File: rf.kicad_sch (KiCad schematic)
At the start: 10 parts, among them Q1 2N7002

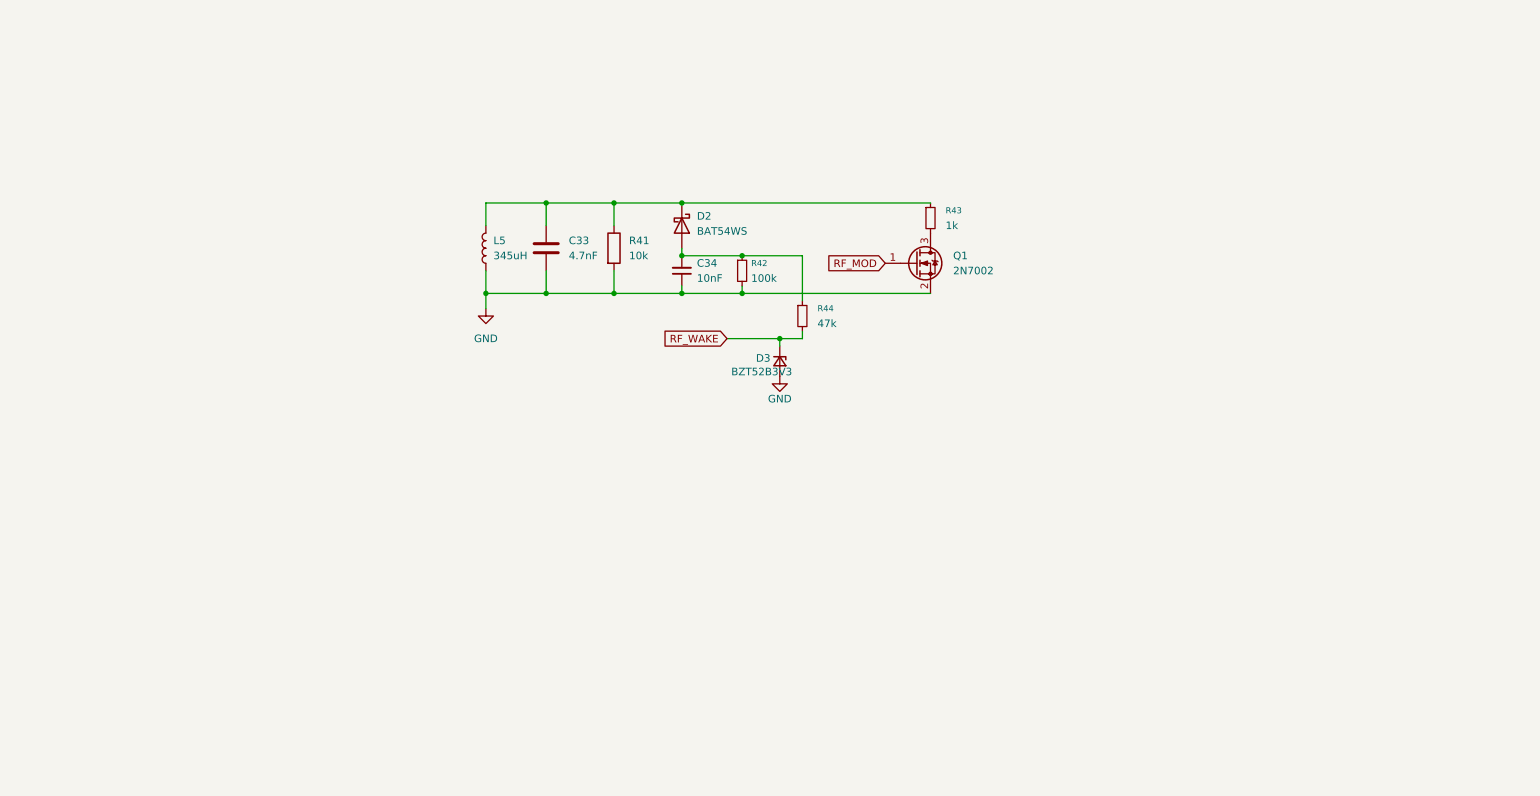
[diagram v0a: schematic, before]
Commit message: finish up everything but nfc
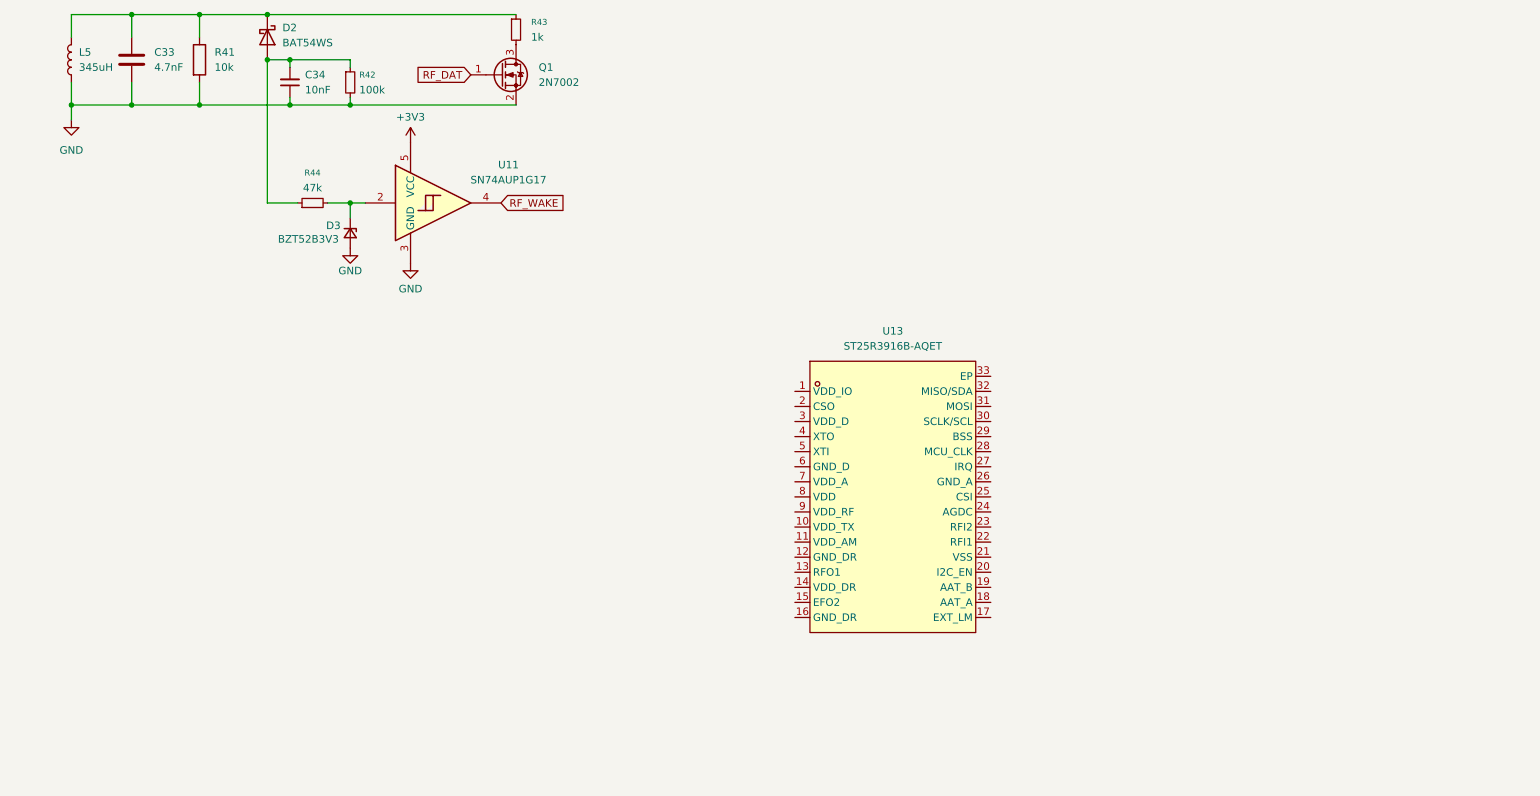
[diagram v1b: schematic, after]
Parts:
- added U11: SN74AUP1G17, Package_TO_SOT_SMD:Diodes_SOT-553, symbol 74xGxx:74LVC1G17
- added U13: ST25R3916B-AQET, ST25R3916B-AQET:QFN-32_L5.0-W5.0-P0.50-TL-EP3.5, symbol ST25R3916B-AQET:ST25R3916B-AQET
- C33: LCSC Part (none) -> C1538
- C34: footprint (none) -> Capacitor_SMD:C_0402_1005Metric; LCSC Part (none) -> C15195
- L5: footprint (none) -> custom_footprints:Generic_Solder_Pads_2P; now left out of the parts list
- Q1: LCSC Part (none) -> C8545
- R41: footprint (none) -> Resistor_SMD:R_0402_1005Metric; LCSC Part (none) -> C25744
- R42: footprint (none) -> Resistor_SMD:R_0402_1005Metric; LCSC Part (none) -> C25741
- R43: footprint (none) -> Resistor_SMD:R_0603_1608Metric; LCSC Part (none) -> C21190
- R44: footprint (none) -> Resistor_SMD:R_0402_1005Metric; LCSC Part (none) -> C25792
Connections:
- net GND: now also U11.3 (GND)
- net RF_WAKE: now also U11.4; no longer D3.1 (K), R44.2
- net RF_MOD renamed RF_DAT
- new net: D3.1 (K), R44.2, U11.2
- new net +3V3: U11.5 (VCC)
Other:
- moved on the sheet: C33, C34, D2, L5, Q1, R41, R42, R43, R44

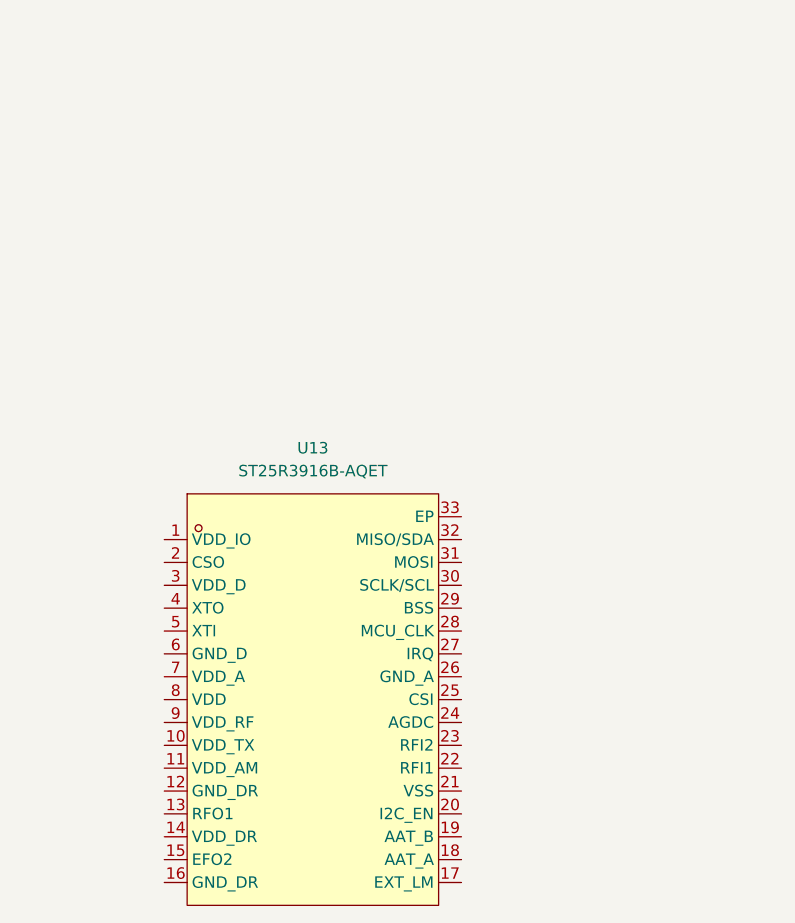
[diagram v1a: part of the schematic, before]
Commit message: progress
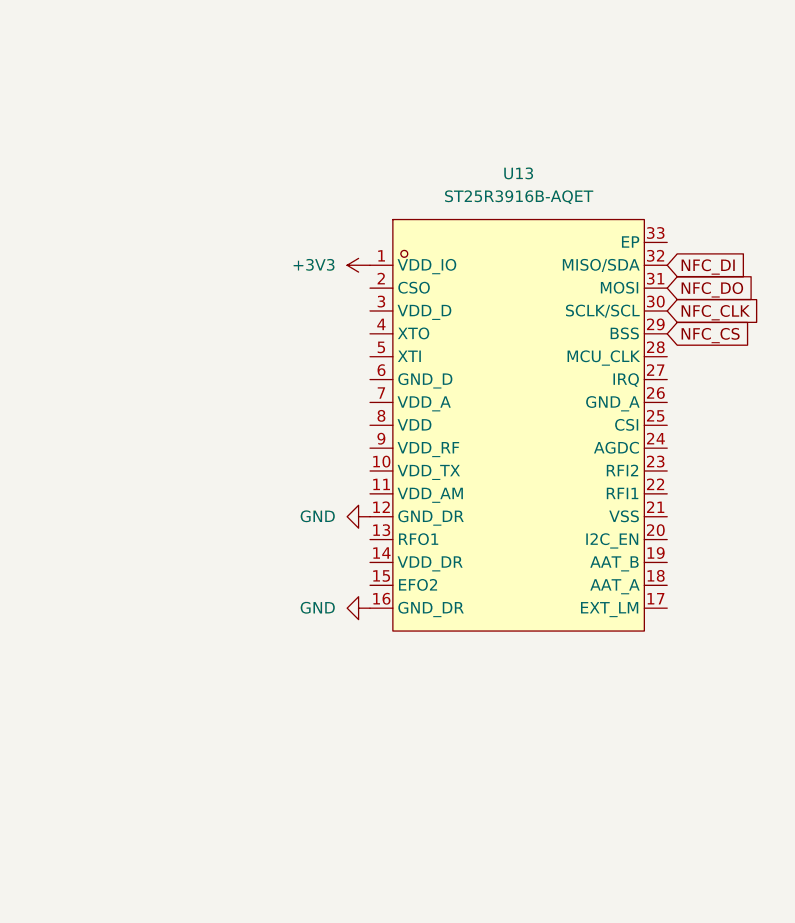
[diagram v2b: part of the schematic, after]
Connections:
- net +3V3: now also U13.1 (VDD_IO)
- net GND: now also U13.12 (GND_DR), U13.16 (GND_DR)
- net NFC_CS: now reaches U13.29 (BSS)
- net NFC_CLK: now reaches U13.30 (SCLK/SCL)
- net NFC_DO: now reaches U13.31 (MOSI)
- net NFC_DI: now reaches U13.32 (MISO/SDA)
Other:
- moved on the sheet: U13

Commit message: push changes before removing fuel gauge
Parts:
- L5: now in the parts list
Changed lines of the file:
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@@
 		(unit 1)
 		(exclude_from_sim no)
-		(in_bom no)
+		(in_bom yes)
 		(on_board yes)
 		(dnp no)

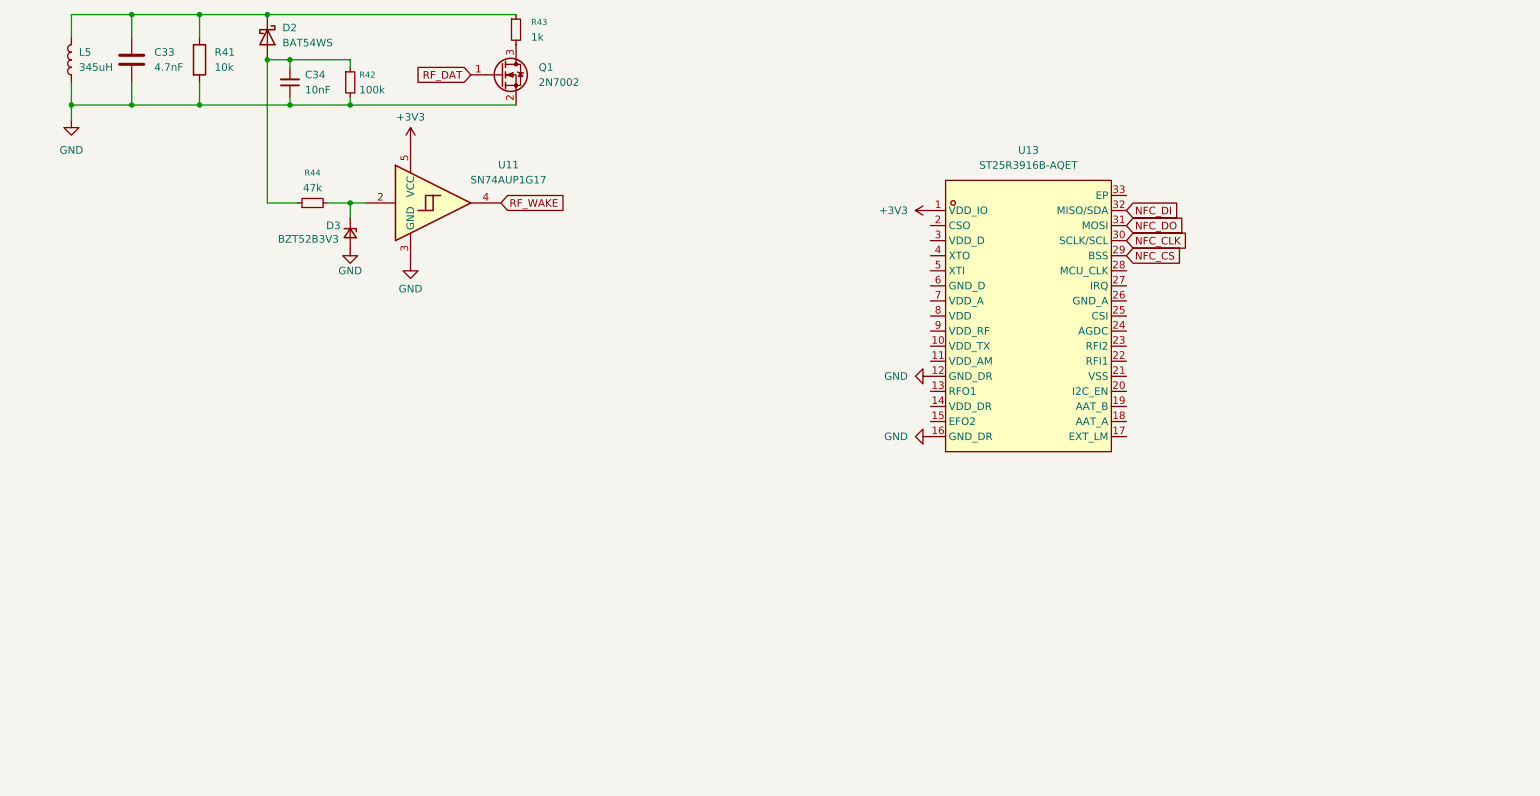
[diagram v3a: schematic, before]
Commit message: hopefully final schematic before splitting out
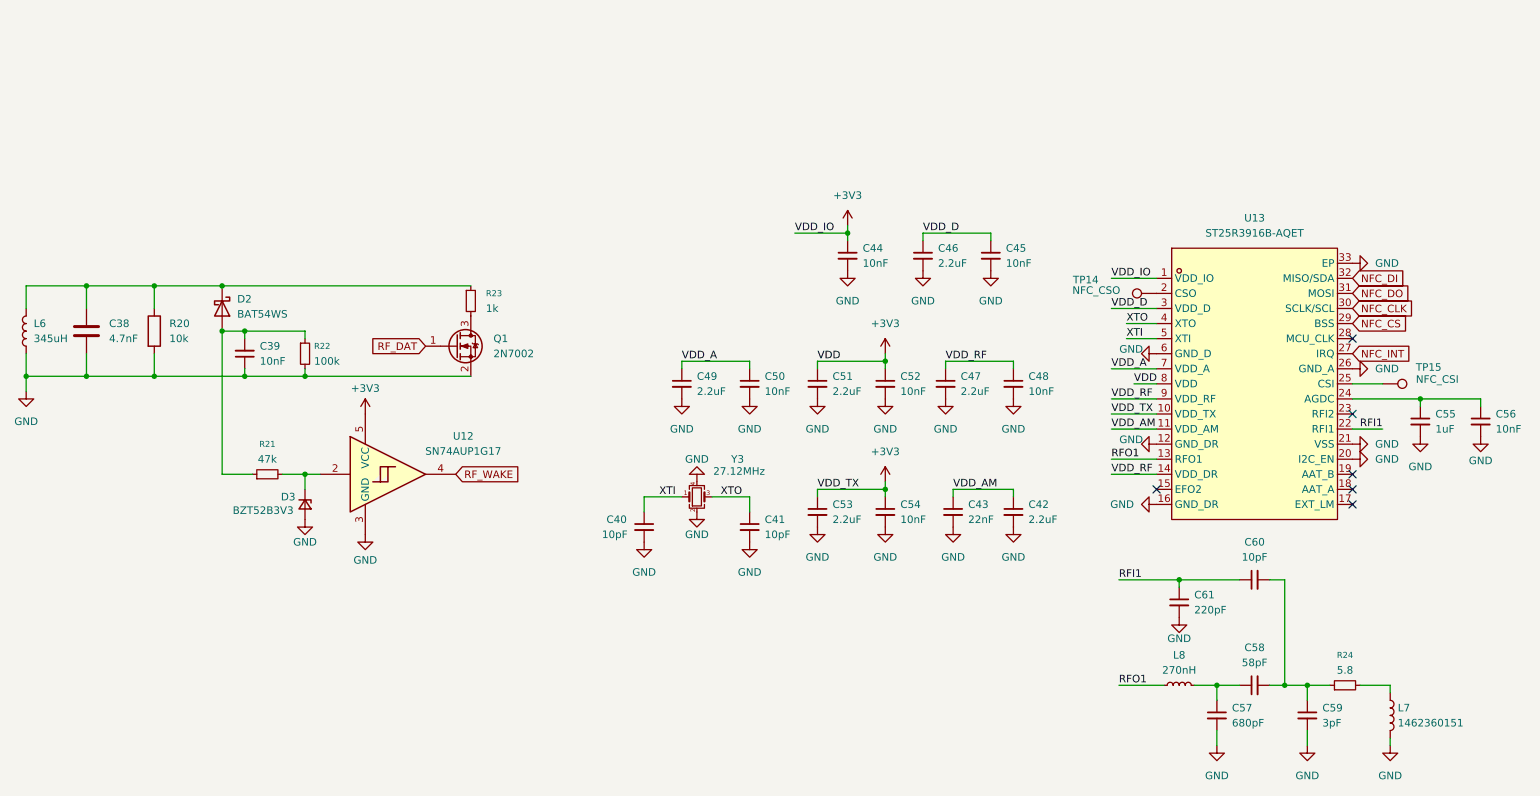
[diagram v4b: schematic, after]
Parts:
- added C40, C41, C60: 10pF, Capacitor_SMD:C_0402_1005Metric, symbol Device:C_Small
- added C42, C46, C47, C49, C51, C53: 2.2uF, Capacitor_SMD:C_0402_1005Metric, symbol Device:C_Small
- added C43: 22nF, Capacitor_SMD:C_0402_1005Metric, symbol Device:C_Small
- added C44, C45, C48, C50, C52, C54, C56: 10nF, Capacitor_SMD:C_0402_1005Metric, symbol Device:C_Small
- added C55: 1uF, Capacitor_SMD:C_0402_1005Metric, symbol Device:C_Small
- added C57: 680pF, Capacitor_SMD:C_0402_1005Metric, symbol Device:C_Small
- added C58: 58pF, Capacitor_SMD:C_0402_1005Metric, symbol Device:C_Small
- added C59: 3pF, Capacitor_SMD:C_0402_1005Metric, symbol Device:C_Small
- added C61: 220pF, Capacitor_SMD:C_0402_1005Metric, symbol Device:C_Small
- added L7: 1462360151, custom_footprints:Generic_Solder_Pads_2P, symbol Device:L
- added L8: 270nH, Inductor_SMD:L_0603_1608Metric, symbol Device:L_Small
- added R24: 5.8, Resistor_SMD:R_0402_1005Metric, symbol Device:R_Small
- added TP14: NFC_CSO, TestPoint:TestPoint_Pad_D1.0mm, symbol Connector:TestPoint
- added TP15: NFC_CSI, TestPoint:TestPoint_Pad_D1.0mm, symbol Connector:TestPoint
- added Y3: 27.12MHz, Crystal:Crystal_SMD_2016-4Pin_2.0x1.6mm, symbol Device:Crystal_GND24_Small
- L6: renamed from L5; now left out of the parts list
- renumbered C33 to C38, C34 to C39, R41 to R20, R44 to R21, R42 to R22, R43 to R23, U11 to U12
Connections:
- net +3V3: now also U13.10 (VDD_TX), U13.8 (VDD), C44.1, C51.1, C52.1, C53.1, C54.1
- net GND: now also U13.20 (I2C_EN), U13.21 (VSS), U13.26 (GND_A), U13.33 (EP), U13.6 (GND_D), C40.2, C41.2, C42.2, C43.2, C44.2, C45.2, C46.2, C47.2, C48.2, C49.2, C50.2, C51.2, C52.2, C53.2, C54.2, C55.2, C56.2, C57.2, C59.2, C61.2, L7.2, Y3.2, Y3.4
- net VDD_AM: now reaches U13.11 (VDD_AM)
- net VDD_AM: now also C42.1, C43.1
- net RFO1: now reaches U13.13 (RFO1)
- net RFO1: now also L8.1
- net VDD_RF: now reaches U13.14 (VDD_DR)
- net VDD_RF: now also U13.9 (VDD_RF), C47.1, C48.1
- net at U13.2 (CSO): now also TP14.1
- net RFI1: now reaches U13.22 (RFI1)
- net RFI1: now also C60.1, C61.1
- net at U13.24 (AGDC): now also C55.1, C56.1
- net at U13.25 (CSI): now also TP15.1
- net NFC_INT: now reaches U13.27 (IRQ)
- net VDD_D: now reaches U13.3 (VDD_D)
- net VDD_D: now also C45.1, C46.1
- net XTO: now reaches U13.4 (XTO)
- net XTO: now also C41.1, Y3.3
- net XTI: now reaches U13.5 (XTI)
- net XTI: now also C40.1, Y3.1
- net VDD_A: now reaches U13.7 (VDD_A)
- net VDD_A: now also C49.1, C50.1
- new net: C57.1, C58.1, L8.2
- new net: C58.2, C59.1, C60.2, R24.1
- new net: L7.1, R24.2
- no-connect marks 0 -> 6
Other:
- moved on the sheet: C38, C39, D2, D3, L6, Q1, R20, R21, R22, R23, U12, U13
